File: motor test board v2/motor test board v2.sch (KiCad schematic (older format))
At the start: 8 parts, among them J1 Conn_01x02, J2 Conn_01x07, J3 Conn_01x02, U1 MC33887

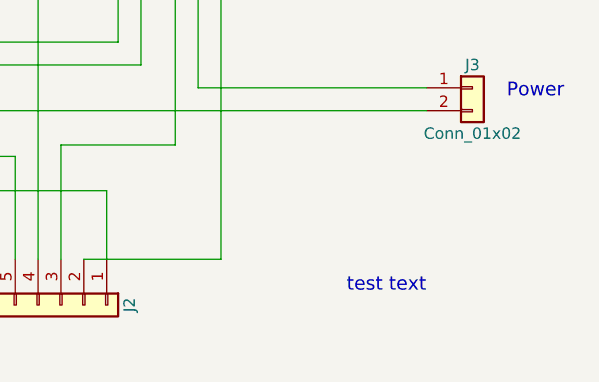
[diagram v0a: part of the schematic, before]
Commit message: removed text
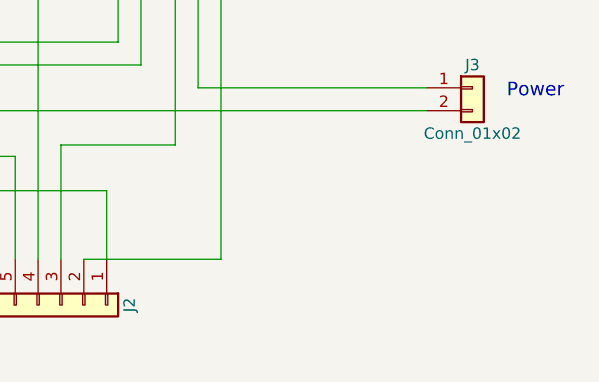
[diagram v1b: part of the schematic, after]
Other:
- note removed: "test text"
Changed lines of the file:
@@
 LIBS:contrib
 LIBS:valves
+LIBS:motor test board-cache
 LIBS:motor test board v2-cache
 EELAYER 25 0
@@
 Text Notes 8100 4900 0    60   ~ 0
 Power\n
-Text Notes 7400 5750 0    60   ~ 0
-test text
 $EndSCHEMATC
